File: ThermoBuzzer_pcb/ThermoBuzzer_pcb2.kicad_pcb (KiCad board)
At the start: 2 copper layers, 61.4 x 58.1 mm, 10 parts, among them SW2 SW_Push

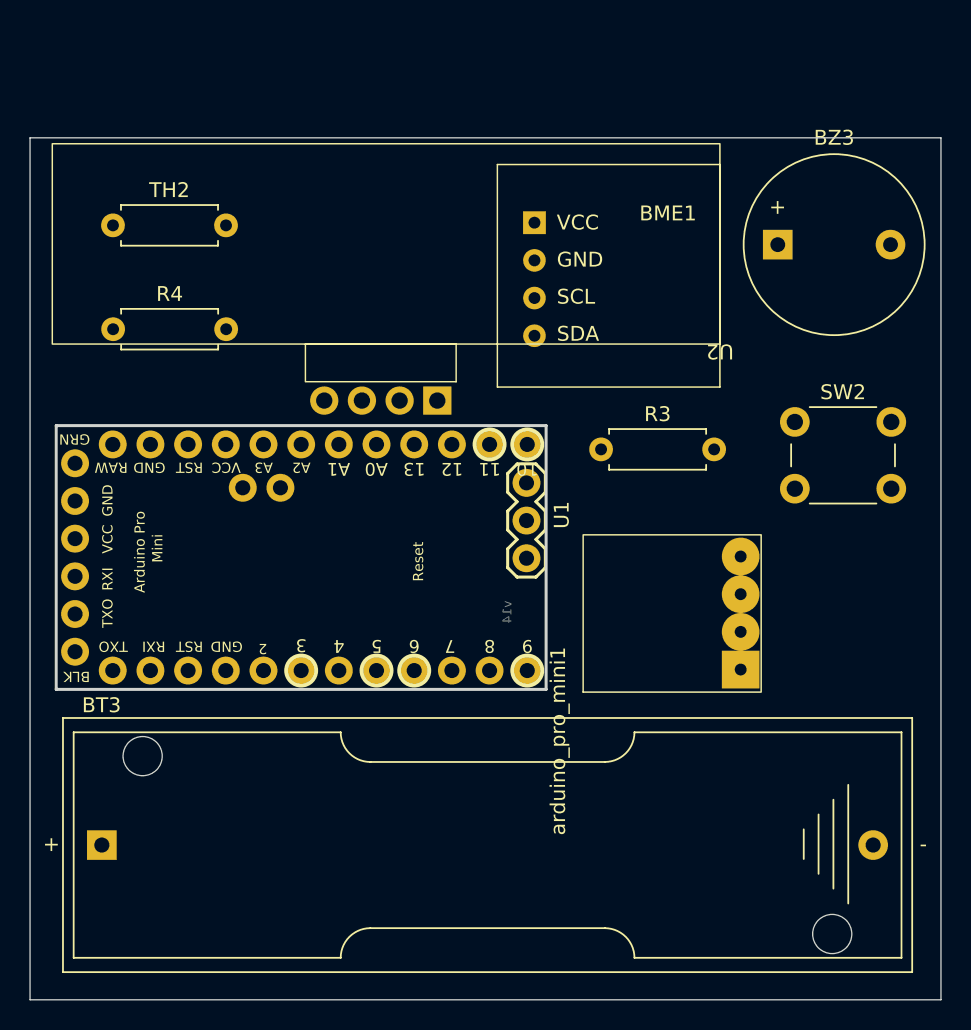
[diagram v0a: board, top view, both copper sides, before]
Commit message: 4.21
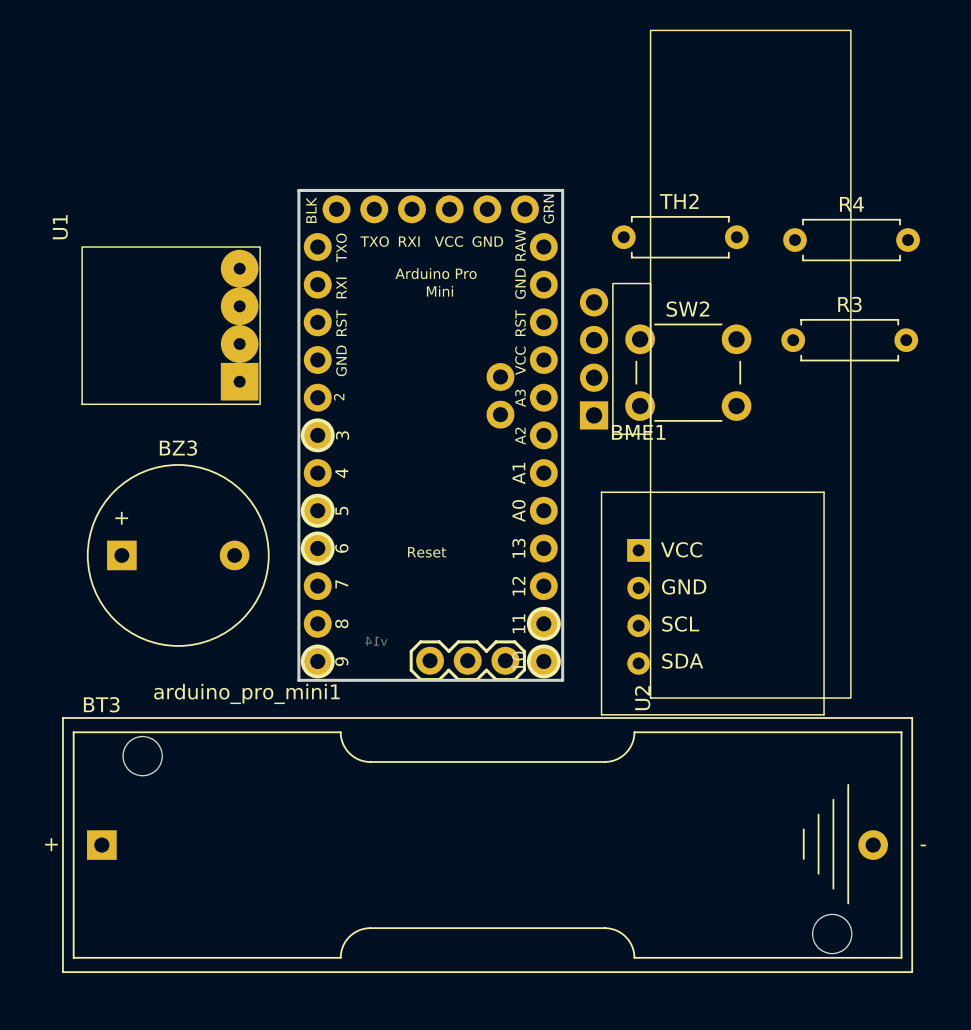
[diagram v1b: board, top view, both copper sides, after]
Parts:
- moved BZ3 48.9 mm to (99.8, 98.0)
- moved R4 46.4 mm to (145.2, 76.8)
- moved U1 38.9 mm to (100.1, 68.6)
- moved TH2 34.4 mm to (133.6, 76.6)
- moved U2 24.3 mm to (135.4, 107.7), turned to 90 degrees
- moved BME1 23.2 mm to (139.1, 101.8)
- moved R3 14.9 mm to (145.0, 83.5)
- moved arduino_pro_mini1 14.1 mm to (113.1, 105.3), turned to 0 degrees
- moved SW2 11.8 mm to (134.7, 83.5)
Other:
- board size 61.4 x 58.1 mm -> 17.8 x 33 mm
